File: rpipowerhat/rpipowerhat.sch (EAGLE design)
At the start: 7 parts, among them U1 OKX-T3-D12, X1 MKDSN1,5/2-5,08, X2 MKDSN1,5/2-5,08

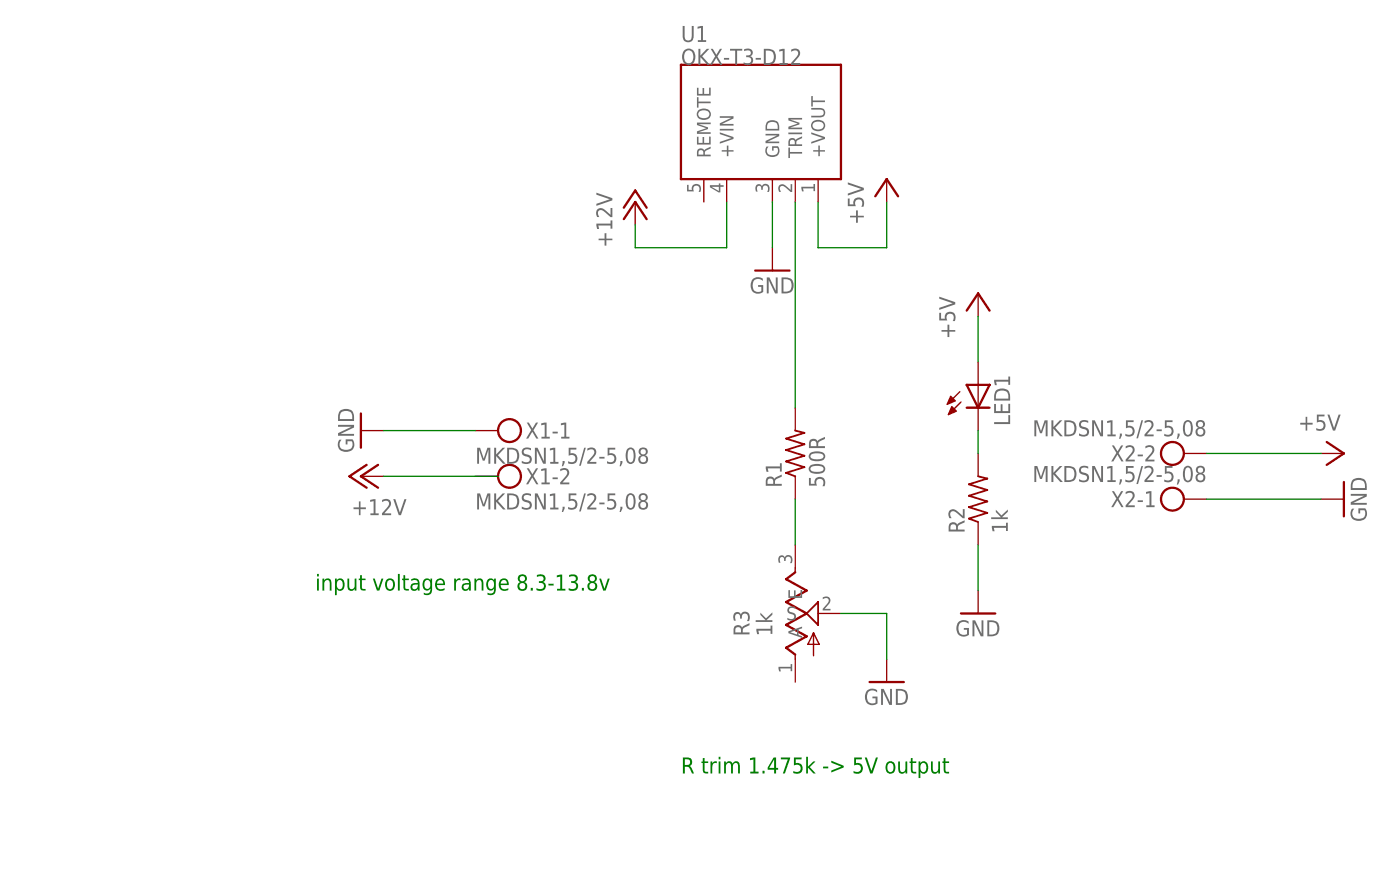
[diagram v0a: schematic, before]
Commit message: homework done
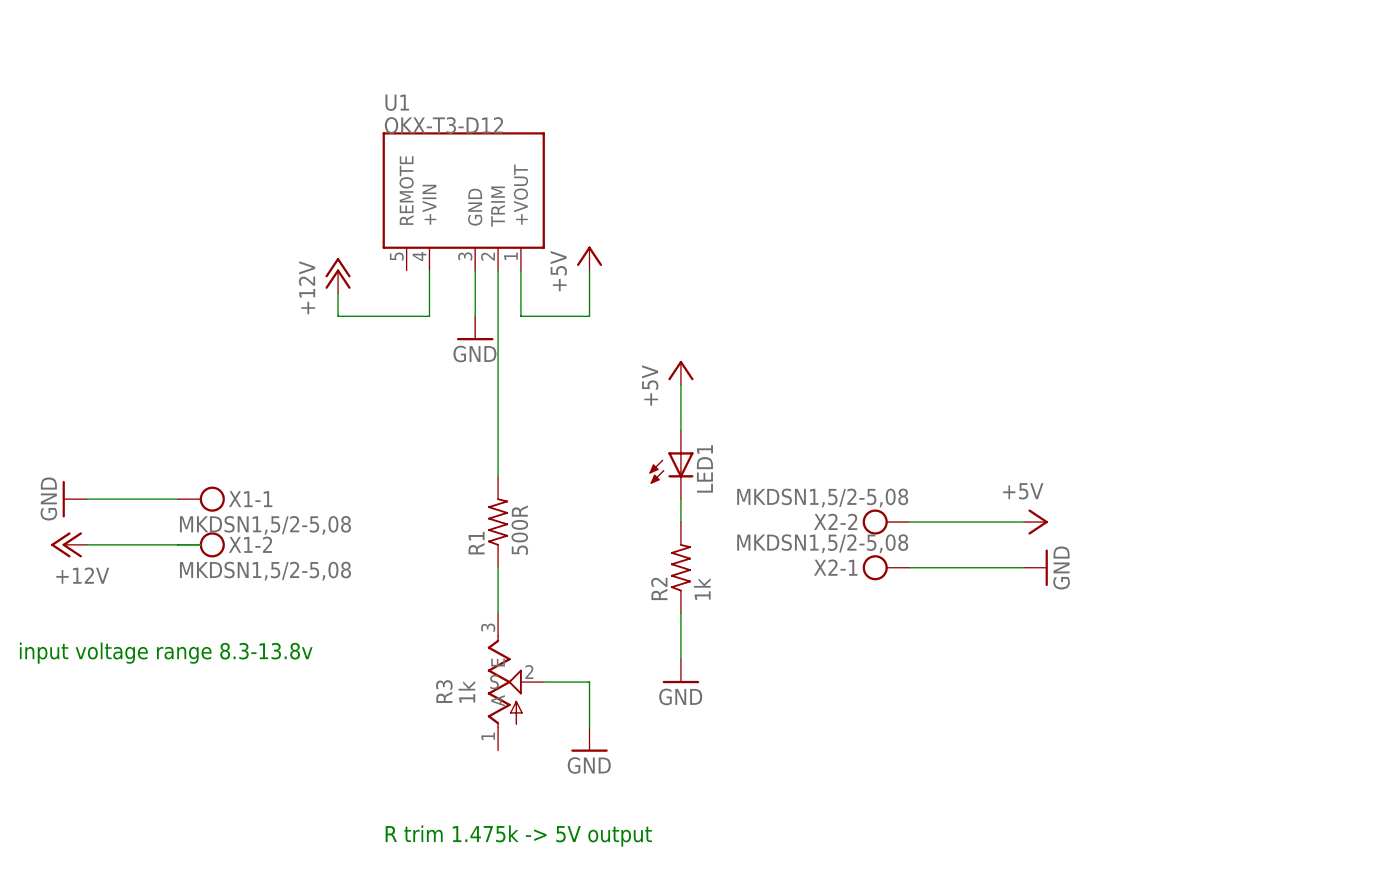
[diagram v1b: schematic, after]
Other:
- moved on the sheet: LED1, R1, R2, R3, U1, X1-1, X1-2, X2-1, X2-2
